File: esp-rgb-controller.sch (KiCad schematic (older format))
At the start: 31 parts, among them J1 Barrel_Jack_Switch, J2 SPARE_GPIO, J3 MCU_UART, J4 AVR-ISP-6, J5 ESP_UART, J6 STRIP, Q1 DMG4800LK3, Q2 DMG4800LK3, Q3 DMG4800LK3, U1 ATmega328P-AU, U2 AP63203WU-7, U3 ESP-01v090

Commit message: initial PCB work
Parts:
- C2: footprint (none) -> Capacitor_SMD:CP_Elec_5x5.3
- C5, C6: footprint (none) -> Capacitor_SMD:CP_Elec_4x4.5
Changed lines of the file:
@@
 F 0 "C2" H 2838 7146 50  0000 L CNN
 F 1 "10uF" H 2838 7055 50  0000 L CNN
-F 2 "" H 2750 7100 50  0001 C CNN
+F 2 "Capacitor_SMD:CP_Elec_5x5.3" H 2750 7100 50  0001 C CNN
 F 3 "~" H 2750 7100 50  0001 C CNN
 	1    2750 7100
@@
 F 0 "C5" H 4550 7350 50  0000 R CNN
 F 1 "22uF" H 4550 7250 50  0000 R CNN
-F 2 "" H 4650 7300 50  0001 C CNN
+F 2 "Capacitor_SMD:CP_Elec_4x4.5" H 4650 7300 50  0001 C CNN
 F 3 "~" H 4650 7300 50  0001 C CNN
 	1    4650 7300
@@
 F 0 "C6" H 4938 7346 50  0000 L CNN
 F 1 "22uF" H 4938 7255 50  0000 L CNN
-F 2 "" H 4850 7300 50  0001 C CNN
+F 2 "Capacitor_SMD:CP_Elec_4x4.5" H 4850 7300 50  0001 C CNN
 F 3 "~" H 4850 7300 50  0001 C CNN
 	1    4850 7300

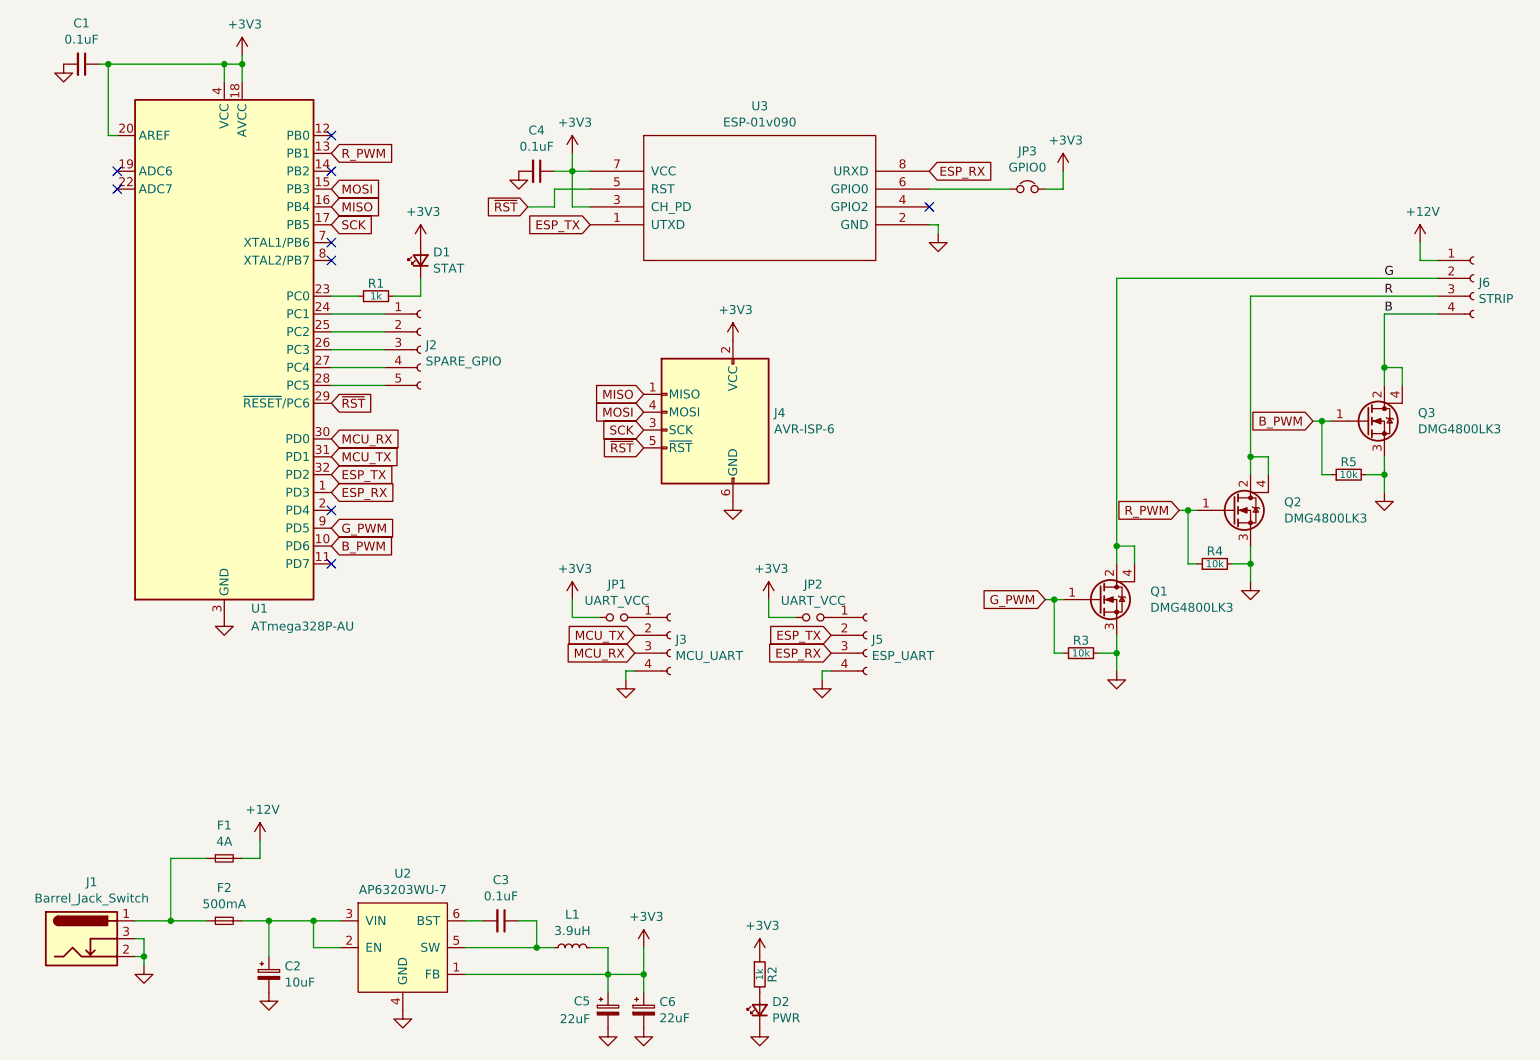
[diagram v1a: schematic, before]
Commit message: more schematic + pcb work
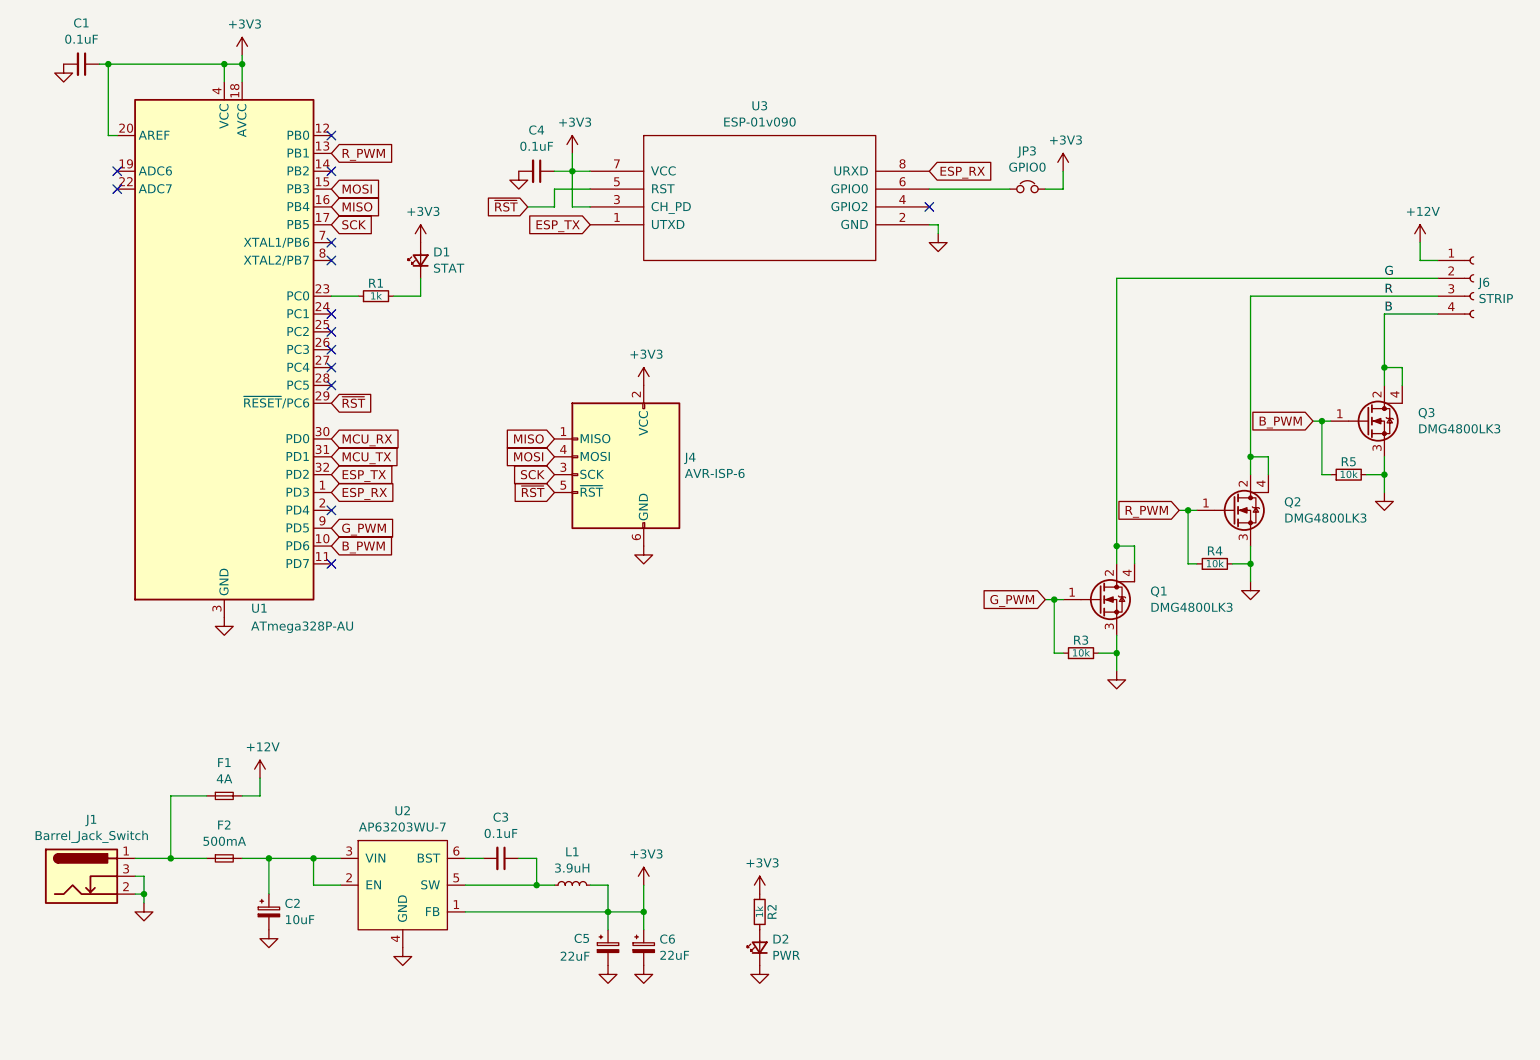
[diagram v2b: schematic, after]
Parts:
- removed J2: SPARE_GPIO, Connector_PinHeader_2.54mm:PinHeader_1x05_P2.54mm_Vertical, symbol Connector:Conn_01x05_Female
- removed J3: MCU_UART, Connector_PinHeader_2.54mm:PinHeader_1x04_P2.54mm_Vertical, symbol Connector:Conn_01x04_Female
- removed J5: ESP_UART, Connector_PinHeader_2.54mm:PinHeader_1x04_P2.54mm_Vertical, symbol Connector:Conn_01x04_Female
- removed JP1, JP2: UART_VCC, Connector_PinHeader_2.54mm:PinHeader_1x02_P2.54mm_Vertical, symbol Device:Jumper_NO_Small
- J4: footprint Connector_PinHeader_2.54mm:PinHeader_2x03_P2.54mm_Vertical -> Connector_PinHeader_2.54mm:PinHeader_2x03_P2.54mm_Vertical_SMD
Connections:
- no-connect marks 9 -> 14
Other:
- moved on the sheet: C2, C3, C5, C6, D2, F1, F2, J1, J4, L1, R2, U2
